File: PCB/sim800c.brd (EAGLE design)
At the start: 95.2 x 100 mm, 56 parts, among them IC1 ESDA5V3L, IC2 ESDA5V3L, IC3 317T, IC4 317EMP, IC5 ESDA5V3L, J1 USB, J2 Ant GSM, Q1 BC846, Q2 BC846, Q3 BC846, Q4 BC846

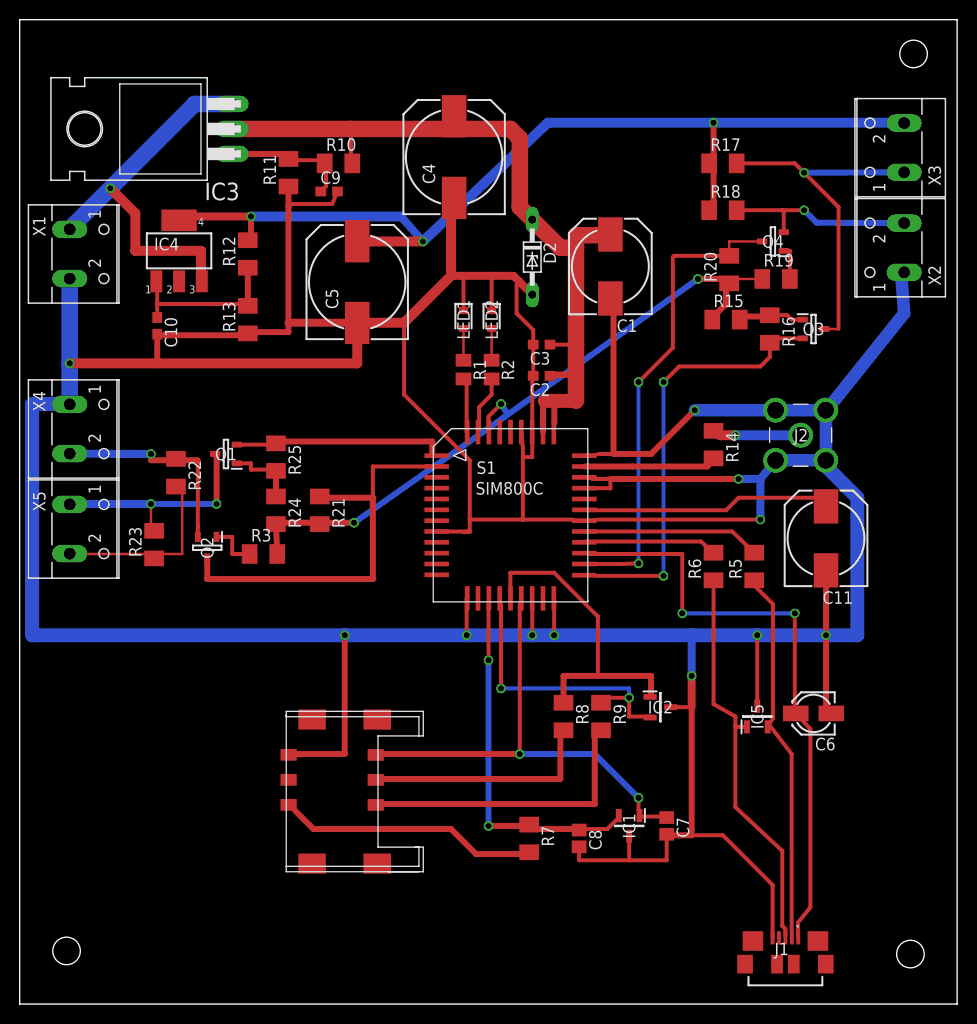
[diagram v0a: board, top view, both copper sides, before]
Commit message: Add files via upload
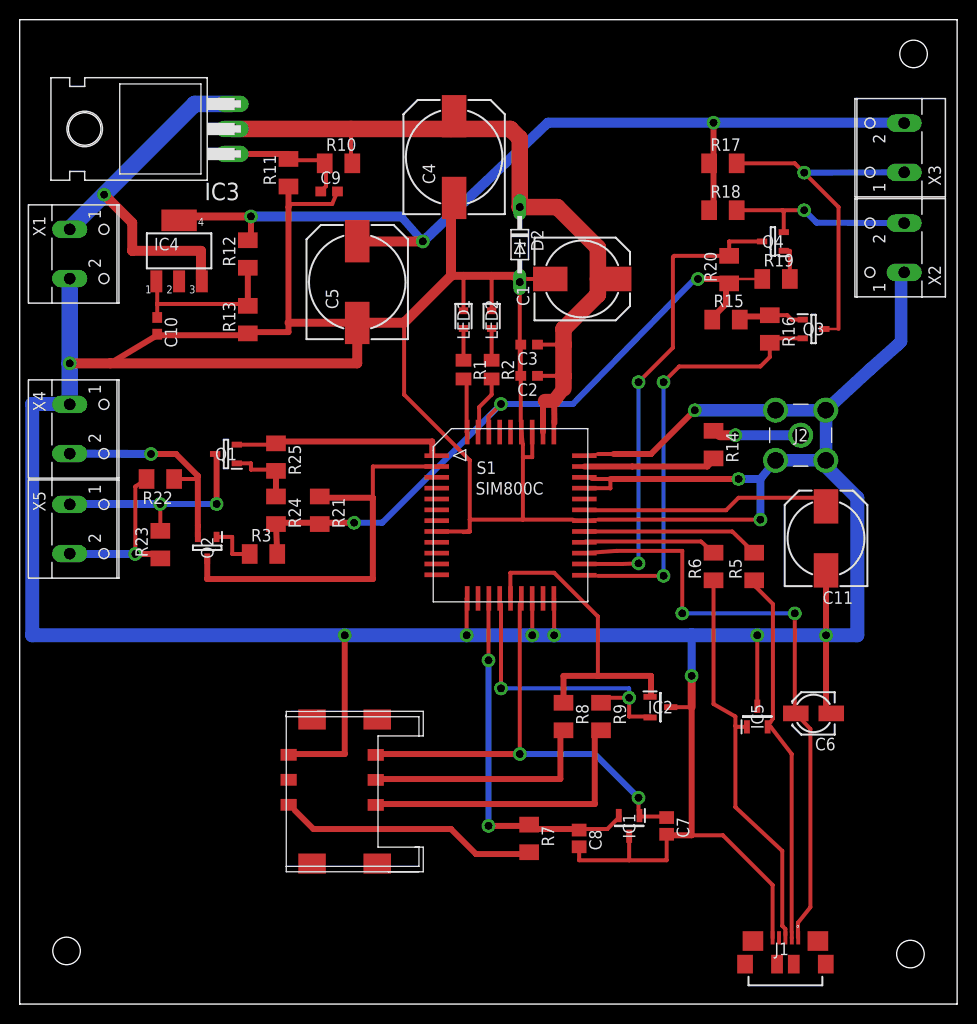
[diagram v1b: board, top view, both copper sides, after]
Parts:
- moved C1 3.13 mm to (57.1, 73.7), turned to 0 degrees
- moved D2 1.80 mm to (50.8, 77.2)
- moved R22 1.71 mm to (14.3, 53.3), turned to 180 degrees
- moved C2 1.27 mm to (51.8, 63.8)
- moved C3 1.27 mm to (51.8, 67.0)
- moved R23 0.63 mm to (14.3, 46.7)
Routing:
- net GND: track 528.6 -> 521.6 mm
- net +5V: track 88.5 -> 83.4 mm
- net N$37: track 4.76 -> 0.00 mm
- net N$38: track 19.1 -> 20.6 mm, vias 0 -> 1
- net N$31: track 21.6 -> 22.9 mm
- net N$16: track 44.9 -> 43.8 mm
- net N$30: track 70.4 -> 71.3 mm
